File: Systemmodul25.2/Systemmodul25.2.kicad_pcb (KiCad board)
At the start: 2 copper layers, 61 x 116.8 mm, 33 parts, among them J1 DIN41612_02x16_AB, J2 DIN41612_02x16_AB, J3 AVR-ISP-6, Q1 12.00J1, U1 W27E040, U2 W27E040, U3 M48T18-100PC1, U4 ATmega8515-16A, U5 MAX690xPA

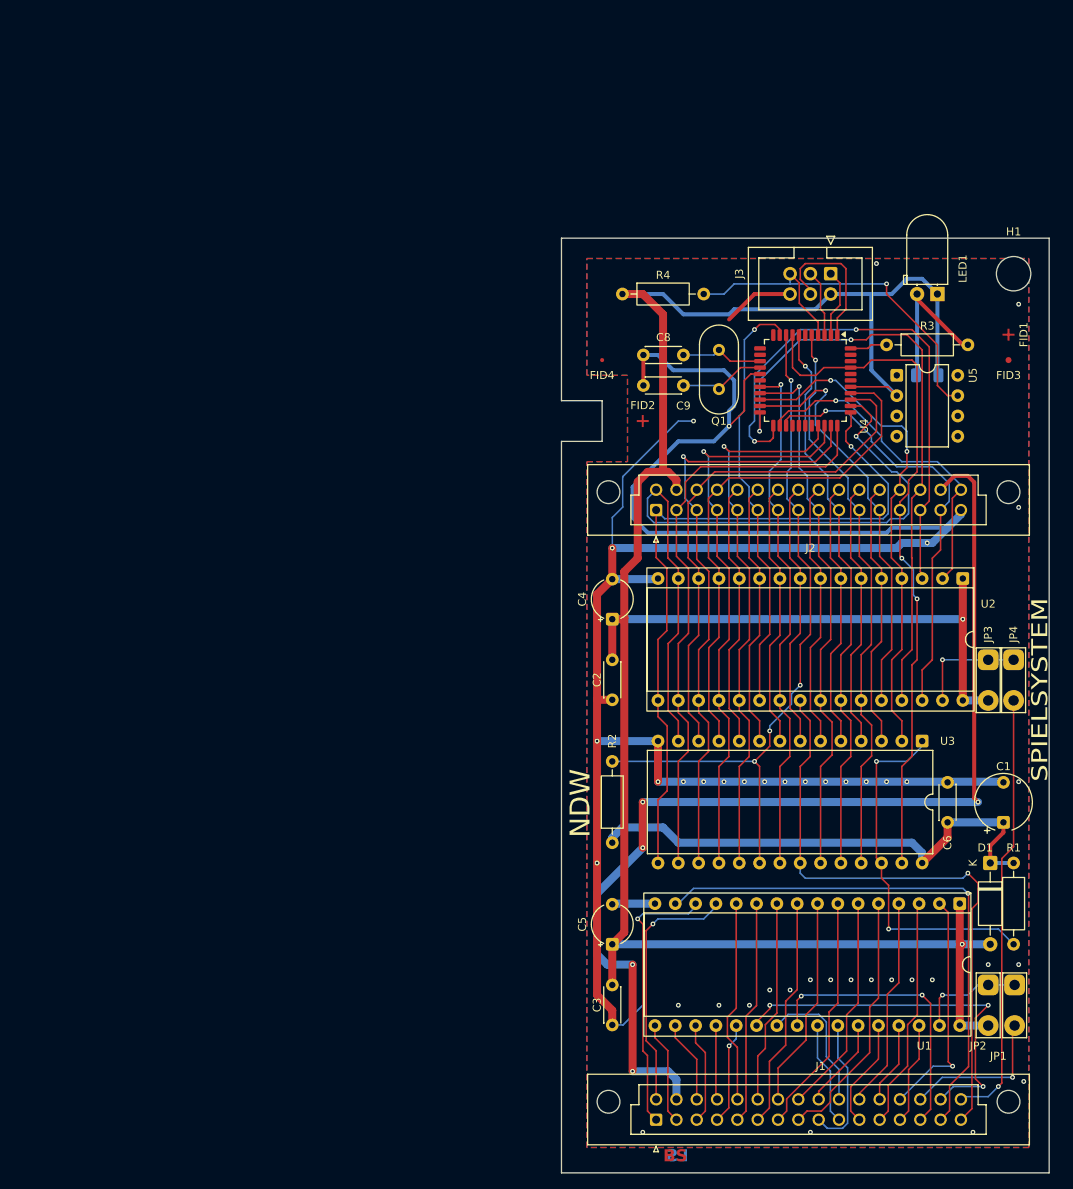
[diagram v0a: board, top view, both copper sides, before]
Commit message: move board
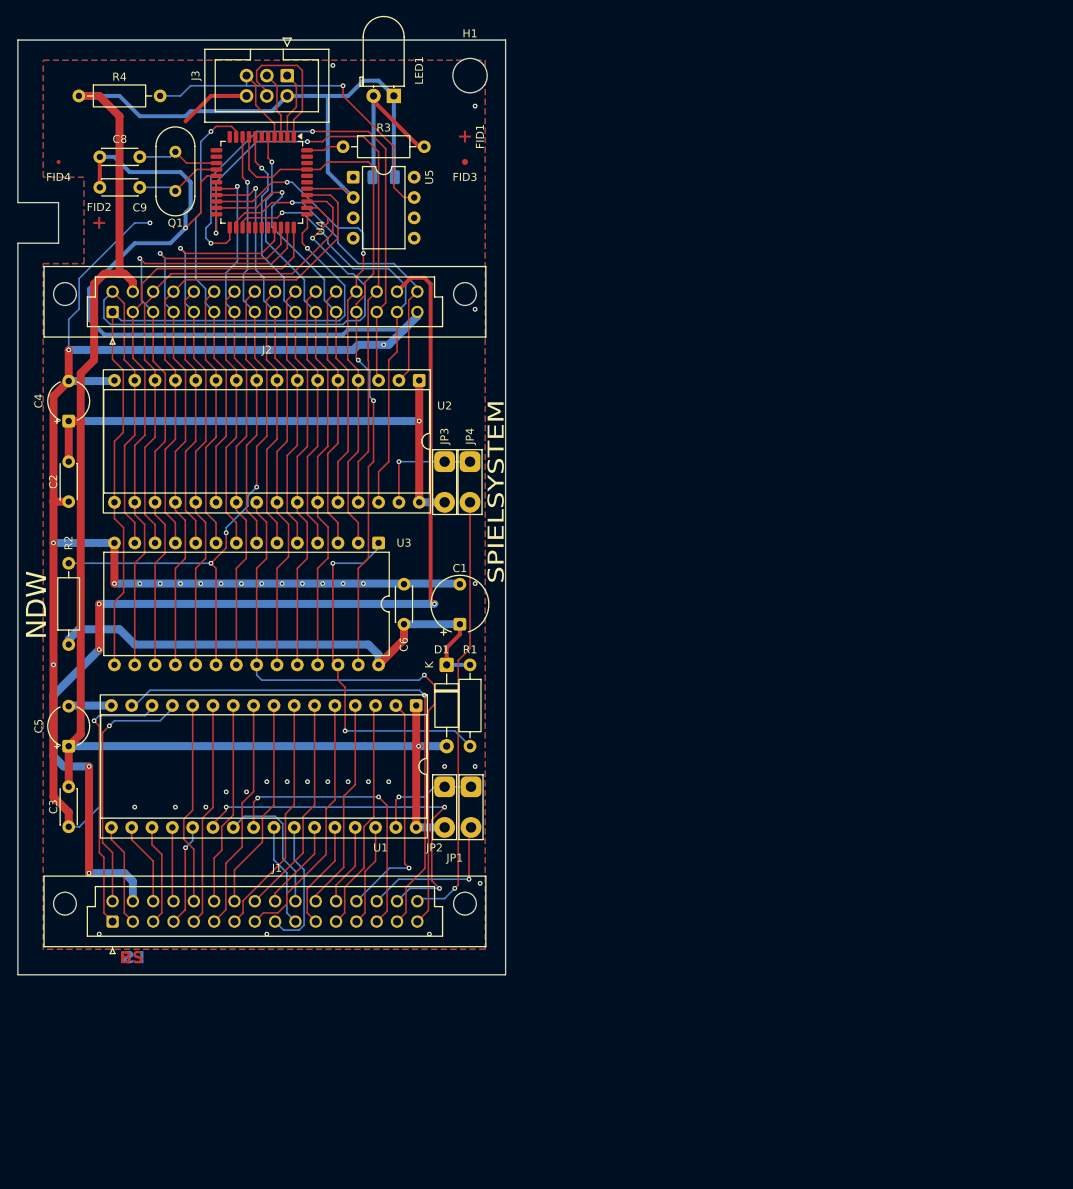
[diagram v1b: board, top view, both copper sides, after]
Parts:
- moved C2 72.3 mm to (21.0, 67.3)
- moved C3 72.3 mm to (21.0, 108.0)
- moved C4 72.3 mm to (21.0, 62.2)
- moved C5 72.3 mm to (21.0, 102.9)
- moved C8 72.3 mm to (24.8, 29.2)
- moved C9 72.3 mm to (24.8, 33.0)
- moved D1 72.3 mm to (68.2, 92.7)
- moved FID1 72.3 mm to (70.5, 26.7)
- moved FID3 72.3 mm to (70.5, 29.8)
- moved JP1 72.3 mm to (71.2, 108.0)
- moved LED2 72.3 mm to (60.3, 31.8)
- moved R2 72.3 mm to (21.0, 90.2)
- moved U1 72.3 mm to (64.4, 97.8)
- moved U2 72.3 mm to (64.8, 57.1)
- moved U3 72.3 mm to (59.7, 77.5)
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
